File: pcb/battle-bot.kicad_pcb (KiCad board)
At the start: 4 copper layers, 99.2 x 51.2 mm, 219 parts, among them J1 Conn_01x02_Pin, J2 Conn_01x04_MountingPin, Q1 AON7544, Q2 AO3401A, Q21 GANE3R9, Q22 GANE3R9, Q23 GANE3R9, Q24 GANE3R9, Q25 GANE3R9, Q26 GANE3R9, Q27 AON7544, Q28 AON7544, Q29 AON7544, Q30 AON7544, Q31 AON7544, Q32 AON7544, Q33 AON7544, Q34 AON7544, Q35 AON7544, Q36 AON7544, Q37 AON7544, Q38 AON7544, Q39 AON7544, Q40 AON7544, Q41 AON7544, Q42 AON7544, Q43 AON7544, U1 TPS53319, U10 LMG1205, U11 LMG1205, U12 LMG1205, U13 ACS780xLRTR-100B, U15 LP38690SD, U2 nRF24L01P, U3 AT2401C, U4 ICM-42688-P, U5 LFL152G45TC1A219, U6 STM32G431RBTx, U7 DRV8323H, U8 DRV8323H, U9 DRV8323H, Y1 16MHz

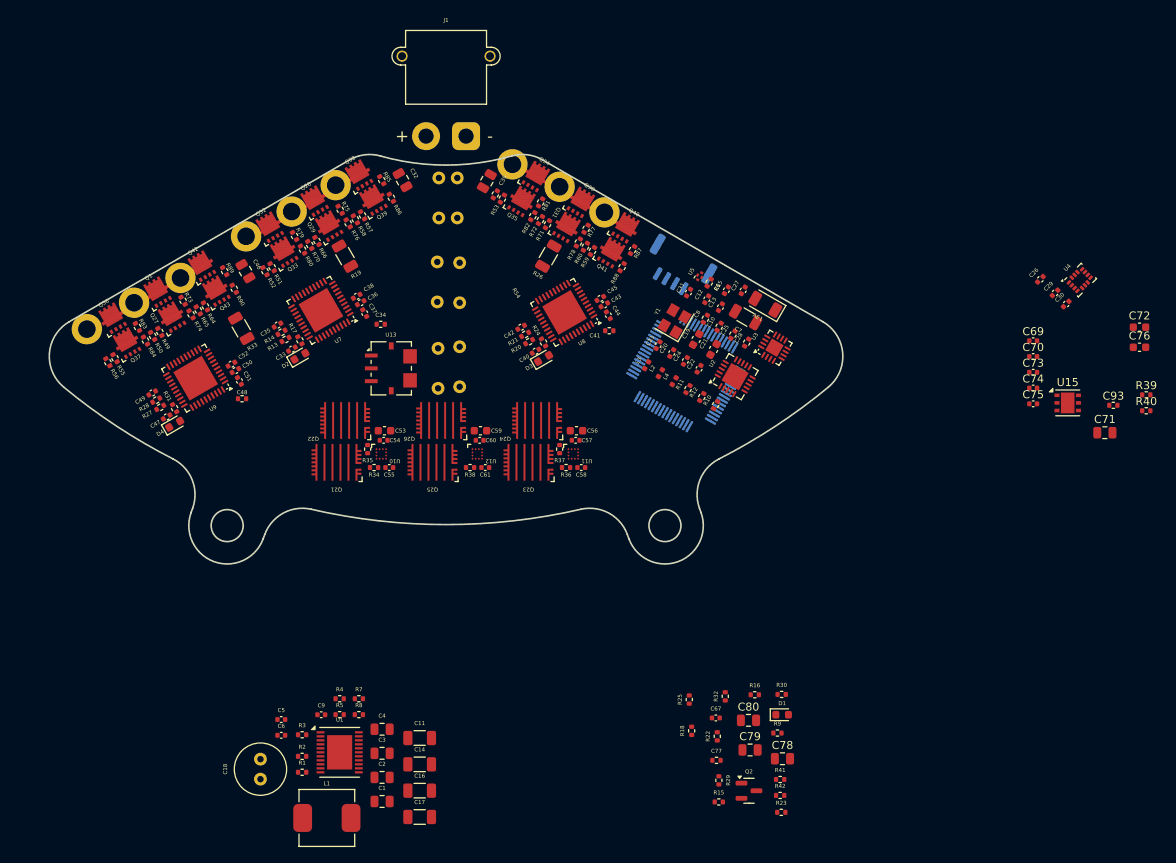
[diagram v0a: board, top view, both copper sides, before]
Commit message: Save layout
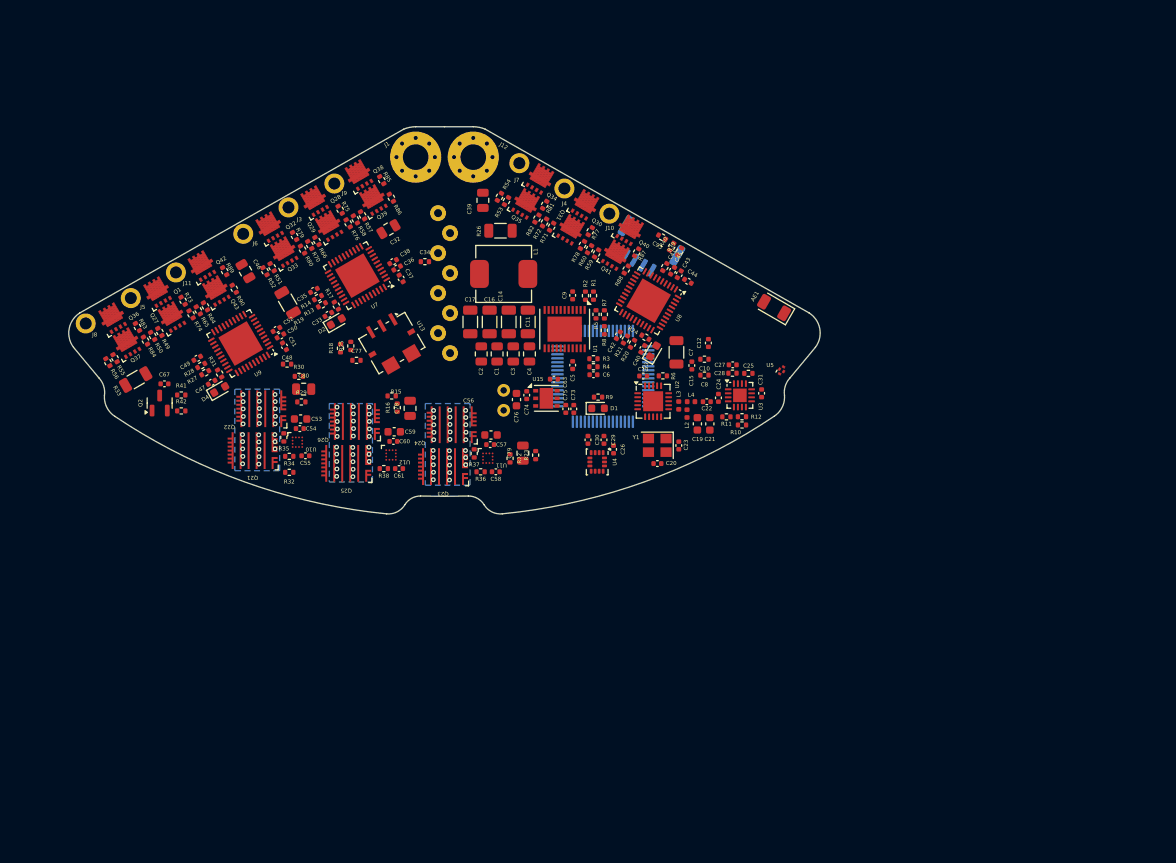
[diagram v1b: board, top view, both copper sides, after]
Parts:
- removed ? (x3): , 
- removed the C68 at (99.2, 54.9)
- removed the C68 at (99.1, 44.1)
- removed the C68 at (101.9, 49.2)
- removed the C68 at (101.9, 59.7)
- removed the C68 at (99.3, 33.6)
- removed C69, C70: 100n, Capacitor_SMD:C_0402_1005Metric
- removed C71: 22u, Capacitor_SMD:C_0805_2012Metric
- removed C72: 22u, Capacitor_SMD:C_0603_1608Metric
- removed REF** (x6): MountingHole_2.2mm_M2_DIN965_Pad, MountingHole:MountingHole_2.2mm_M2_DIN965_Pad
- added C62: 2m2, User_Footprints:C_D10xL16_Horizontal, B.Cu at (100.7, 40.5)
- added C63: 100n, Capacitor_SMD:C_0402_1005Metric, F.Cu at (113.7, 58.8)
- added C65: 2m2, User_Footprints:C_D10xL16_Horizontal, B.Cu at (99.2, 53.0)
- added C66: 2m2, User_Footprints:C_D10xL16_Horizontal, B.Cu at (100.7, 50.5)
- added J10: Conn_01x01_Pin, User_Footprints:Pad-P1.5, F.Cu at (120.6, 38.1)
- added J11: Conn_01x01_Pin, User_Footprints:Pad-P1.5, F.Cu at (66.4, 45.4)
- added J12: Conn_01x01_Pin, MountingHole:MountingHole_3.2mm_M3_Pad_Via, F.Cu at (103.6, 31.0)
- added J3: Conn_01x01_Pin, User_Footprints:Pad-P1.5, F.Cu at (80.5, 37.3)
- added J4: Conn_01x01_Pin, User_Footprints:Pad-P1.5, F.Cu at (115.0, 34.9)
- added J5: Conn_01x01_Pin, User_Footprints:Pad-P1.5, F.Cu at (60.8, 48.6)
- added J6: Conn_01x01_Pin, User_Footprints:Pad-P1.5, F.Cu at (74.8, 40.6)
- added J7: Conn_01x01_Pin, User_Footprints:Pad-P1.5, F.Cu at (109.4, 31.8)
- added J8: Conn_01x01_Pin, User_Footprints:Pad-P1.5, F.Cu at (55.2, 51.8)
- added J9: Conn_01x01_Pin, User_Footprints:Pad-P1.5, F.Cu at (86.2, 34.3)
- AE1: value Antenna -> Antenna_Chip
- C18: moved to B.Cu
- C68: footprint Capacitor_THT:C_Radial_D10.0mm_H16.0mm_P5.00mm -> User_Footprints:C_D10xL16_Horizontal
- J1: value Conn_01x02_Pin -> Conn_01x01_Pin; footprint Connector_AMASS:AMASS_XT30PW-M_1x02_P2.50mm_Horizontal -> MountingHole:MountingHole_3.2mm_M3_Pad_Via
- moved R41 89.0 mm to (67.1, 60.7)
- moved R42 89.0 mm to (67.1, 62.7)
- moved Q2 88.2 mm to (64.4, 61.7), turned to 90 degrees
- moved C67 80.6 mm to (65.0, 59.3)
- moved C76 78.2 mm to (109.0, 61.3), turned to -90 degrees
- moved R30 72.3 mm to (81.8, 58.4)
- moved L1 71.5 mm to (107.4, 45.6), turned to 180 degrees
- moved R29 70.4 mm to (82.1, 61.6), turned to 0 degrees
- moved R1 69.8 mm to (118.6, 48.3), turned to 90 degrees
- moved C80 69.3 mm to (82.4, 60.0)
- moved R2 67.6 mm to (117.6, 48.3), turned to -90 degrees
- moved C77 67.3 mm to (89.0, 56.4)
- moved R15 65.2 mm to (93.4, 60.9), turned to 180 degrees
- moved U15 65.2 mm to (112.7, 61.1)
- moved R18 64.9 mm to (87.0, 54.9)
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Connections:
- AE1 pad 2: (no net) -> unconnected-(AE1-PCB_Trace-Pad2)
- C68 pad 1: VDD -> GND
- C68 pad 2: GND -> VDD
- J1 pad 1: VDD -> GND
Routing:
- net /LargeMotor/OUTC: vias 0 -> 28
- net /LargeMotor/OUTB: vias 0 -> 28
- net /LargeMotor/OUTA: vias 0 -> 28
- added copper zone on B.Cu, net /LargeMotor/OUTA
- added copper zone on B.Cu, net /LargeMotor/OUTB
- added copper zone on B.Cu, net /LargeMotor/OUTC
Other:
- board size 99.2 x 51.2 mm -> 93.9 x 48.4 mm
- board text added: "Please Don't Explode 9000"

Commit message: Save old buck regulator
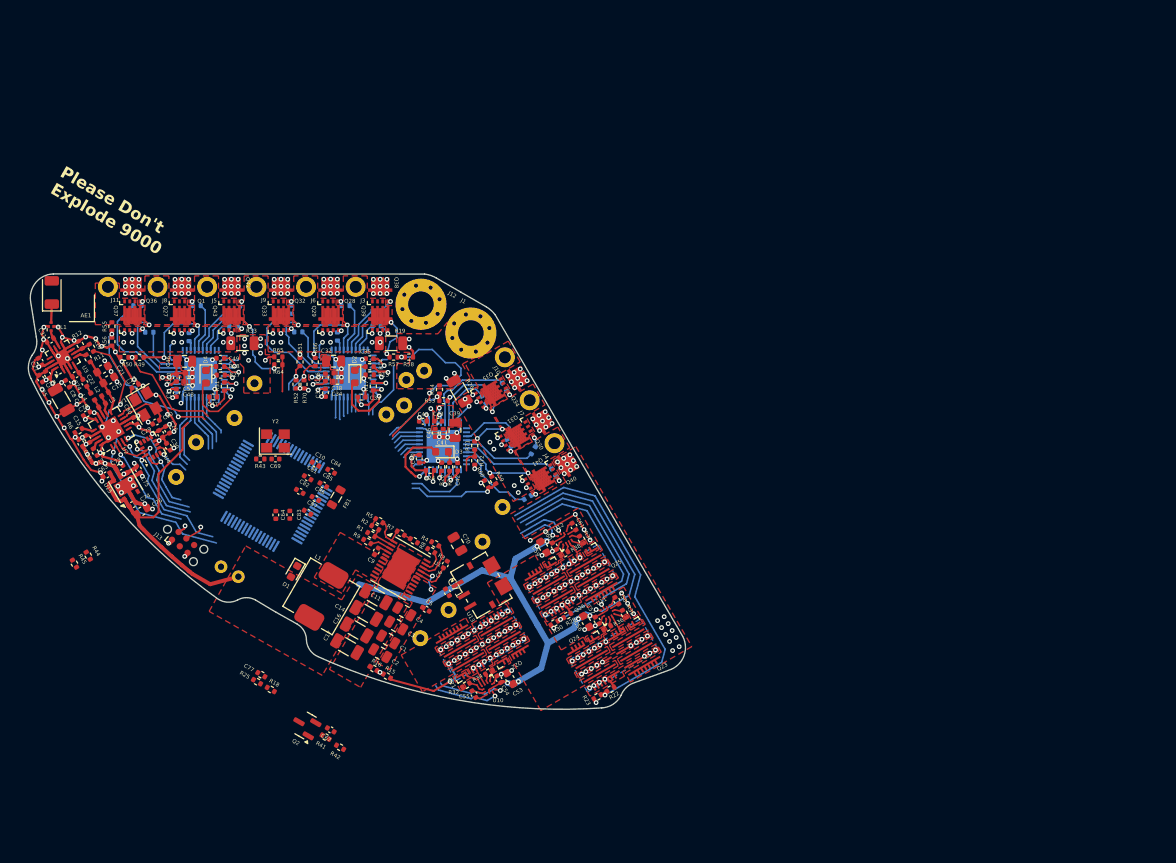
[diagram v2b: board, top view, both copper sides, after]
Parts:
- removed C93: 10u, Resistor_SMD:R_0402_1005Metric
- removed J2: Conn_01x04_MountingPin, Connector_JST:JST_GH_SM04B-GHS-TB_1x04-1MP_P1.25mm_Horizontal
- removed R39, R40: 2k2, Resistor_SMD:R_0402_1005Metric
- added C64: 12p, Capacitor_SMD:C_0402_1005Metric, F.Cu at (78.9, 75.7)
- added C69: 12p, Capacitor_SMD:C_0402_1005Metric, F.Cu at (78.9, 68.7)
- added C70: 22u, Capacitor_SMD:C_0805_2012Metric, F.Cu at (101.6, 79.3)
- added C71: 100n, Capacitor_SMD:C_0402_1005Metric, F.Cu at (100.4, 85.4)
- added C72: 2m2, User_Footprints:C_D10xL16_Horizontal, B.Cu at (104.7, 79.1)
- added C81: 100n, Capacitor_SMD:C_0402_1005Metric, F.Cu at (82.9, 71.1)
- added C82: 100n, Capacitor_SMD:C_0402_1005Metric, F.Cu at (81.9, 72.8)
- added C83: 100n, Capacitor_SMD:C_0402_1005Metric, F.Cu at (80.7, 75.7)
- added C84: 100n, Capacitor_SMD:C_0402_1005Metric, F.Cu at (85.8, 70.3)
- added C85: 1u, Capacitor_SMD:C_0402_1005Metric, F.Cu at (84.8, 72.0)
- added C86: 1u, Capacitor_SMD:C_0402_1005Metric, F.Cu at (83.9, 73.7)
- added C87: 100n, Capacitor_SMD:C_0402_1005Metric, F.Cu at (82.9, 75.4)
- added FB1: FerriteBead, Inductor_SMD:L_0805_2012Metric, F.Cu at (86.5, 73.5)
- added J13: Conn_ARM_SWD_TagConnect_TC2030-NL, Connector:Tag-Connect_TC2030-IDC-NL_2x03_P1.27mm_Vertical, F.Cu at (67.3, 79.2)
- added R43: 1k, Resistor_SMD:R_0402_1005Metric, F.Cu at (77.0, 68.7)
- added R44: 15k, Resistor_SMD:R_0402_1005Metric, F.Cu at (55.5, 80.8)
- added R45: 2k2, Resistor_SMD:R_0402_1005Metric, F.Cu at (53.7, 81.8)
- added Y2: 16MHz, Crystal:Crystal_SMD_3225-4Pin_3.2x2.5mm, F.Cu at (78.9, 66.5)
- C10: value 100n -> 10u; footprint Resistor_SMD:R_0402_1005Metric -> Capacitor_SMD:C_0402_1005Metric
- C25, C28: footprint Resistor_SMD:R_0402_1005Metric -> Capacitor_SMD:C_0402_1005Metric
- C67: value C -> 4u7
- C7: footprint Resistor_SMD:R_1206_3216Metric -> Capacitor_SMD:C_1206_3216Metric
- C78: value 22u -> 2m2; footprint Capacitor_SMD:C_0805_2012Metric -> User_Footprints:C_D10xL16_Horizontal; moved to B.Cu
- C79, C80: value 22u -> 10n; footprint Capacitor_SMD:C_0805_2012Metric -> Capacitor_SMD:C_0402_1005Metric
- C8: value 10u -> 1u; footprint Resistor_SMD:R_0402_1005Metric -> Capacitor_SMD:C_0402_1005Metric
- R1: value 22k -> 47k
- R15, R22, R29: value 4k7 -> 10k
- R16, R23, R30: value 1k -> 1k5
- R2: value 10k -> 4k7
- R42: value R -> 100k
- R73, R74, R75, R76, R77, R78, R79, R80, R81, R82, R83, R84, R85, R86, R87, R88, R89, R90, U7, U8, U9: moved to B.Cu
- moved FL1 91.5 mm to (50.8, 52.2), turned to 90 degrees
- moved AE1 90.3 mm to (50.9, 47.9), turned to 90 degrees
- moved C31 89.2 mm to (50.7, 53.9), turned to -150 degrees
- moved C25 88.5 mm to (49.5, 58.7), turned to 120 degrees
- moved C27 86.6 mm to (49.5, 56.6), turned to 120 degrees
- moved C28 85.6 mm to (50.4, 58.2), turned to 120 degrees
- moved U3 84.8 mm to (52.3, 56.0), turned to 120 degrees
- moved R12 83.2 mm to (54.5, 54.5), turned to 120 degrees
- moved R10 81.9 mm to (55.9, 54.8), turned to -60 degrees
- moved C24 80.4 mm to (53.9, 58.2), turned to -150 degrees
- moved R11 80.1 mm to (55.5, 56.1), turned to 120 degrees
- moved C8 79.6 mm to (52.9, 59.3), turned to -60 degrees
- moved C12 79.4 mm to (54.5, 66.7), turned to 120 degrees
- moved C22 77.8 mm to (55.0, 59.2), turned to 120 degrees
- moved C7 77.1 mm to (52.1, 61.4), turned to -60 degrees
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- renumbered U5 to FL1
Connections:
- C35 pad 1: Net-(U7-VREF) -> +3V3
- C42 pad 1: Net-(U8-VREF) -> +3V3
- C49 pad 1: Net-(U9-VREF) -> +3V3
- C73 pad 1: VDDRF -> +3V3
- C75 pad 1: VDDRF -> +3V3
- C79 pad 1: VDD -> +3V3
- C80 pad 1: VDD -> +3V3
- Q1 pad 1: /SmallMotor3/OUTA -> /SmallMotor3/OUTB
- Q1 pad 2: /SmallMotor3/OUTA -> /SmallMotor3/OUTB
- Q1 pad 3: /SmallMotor3/OUTA -> /SmallMotor3/OUTB
- Q27 pad 5: /SmallMotor3/OUTA -> /SmallMotor3/OUTB
- Q27 pad 6: /SmallMotor3/OUTA -> /SmallMotor3/OUTB
- Q27 pad 7: /SmallMotor3/OUTA -> /SmallMotor3/OUTB
- Q27 pad 8: /SmallMotor3/OUTA -> /SmallMotor3/OUTB
- Q28 pad 1: /SmallMotor1/OUTA -> /SmallMotor1/OUTB
- Q28 pad 2: /SmallMotor1/OUTA -> /SmallMotor1/OUTB
- Q28 pad 3: /SmallMotor1/OUTA -> /SmallMotor1/OUTB
- Q29 pad 5: /SmallMotor1/OUTA -> /SmallMotor1/OUTB
- Q29 pad 6: /SmallMotor1/OUTA -> /SmallMotor1/OUTB
- Q29 pad 7: /SmallMotor1/OUTA -> /SmallMotor1/OUTB
- Q29 pad 8: /SmallMotor1/OUTA -> /SmallMotor1/OUTB
- Q30 pad 1: /SmallMotor2/OUTA -> /SmallMotor2/OUTB
- Q30 pad 2: /SmallMotor2/OUTA -> /SmallMotor2/OUTB
- Q30 pad 3: /SmallMotor2/OUTA -> /SmallMotor2/OUTB
- Q31 pad 5: /SmallMotor2/OUTA -> /SmallMotor2/OUTB
- Q31 pad 6: /SmallMotor2/OUTA -> /SmallMotor2/OUTB
- Q31 pad 7: /SmallMotor2/OUTA -> /SmallMotor2/OUTB
- Q31 pad 8: /SmallMotor2/OUTA -> /SmallMotor2/OUTB
- Q32 pad 1: /SmallMotor1/OUTB -> /SmallMotor1/OUTC
- Q32 pad 2: /SmallMotor1/OUTB -> /SmallMotor1/OUTC
- Q32 pad 3: /SmallMotor1/OUTB -> /SmallMotor1/OUTC
- Q33 pad 5: /SmallMotor1/OUTB -> /SmallMotor1/OUTC
- Q33 pad 6: /SmallMotor1/OUTB -> /SmallMotor1/OUTC
- Q33 pad 7: /SmallMotor1/OUTB -> /SmallMotor1/OUTC
- Q33 pad 8: /SmallMotor1/OUTB -> /SmallMotor1/OUTC
- Q34 pad 1: /SmallMotor2/OUTB -> /SmallMotor2/OUTC
- Q34 pad 2: /SmallMotor2/OUTB -> /SmallMotor2/OUTC
- Q34 pad 3: /SmallMotor2/OUTB -> /SmallMotor2/OUTC
- Q35 pad 5: /SmallMotor2/OUTB -> /SmallMotor2/OUTC
- Q35 pad 6: /SmallMotor2/OUTB -> /SmallMotor2/OUTC
- Q35 pad 7: /SmallMotor2/OUTB -> /SmallMotor2/OUTC
- Q35 pad 8: /SmallMotor2/OUTB -> /SmallMotor2/OUTC
- Q36 pad 1: /SmallMotor3/OUTB -> /SmallMotor3/OUTC
- Q36 pad 2: /SmallMotor3/OUTB -> /SmallMotor3/OUTC
- Q36 pad 3: /SmallMotor3/OUTB -> /SmallMotor3/OUTC
- Q37 pad 5: /SmallMotor3/OUTB -> /SmallMotor3/OUTC
- Q37 pad 6: /SmallMotor3/OUTB -> /SmallMotor3/OUTC
- Q37 pad 7: /SmallMotor3/OUTB -> /SmallMotor3/OUTC
- Q37 pad 8: /SmallMotor3/OUTB -> /SmallMotor3/OUTC
- Q38 pad 1: /SmallMotor1/OUTC -> /SmallMotor1/OUTA
- Q38 pad 2: /SmallMotor1/OUTC -> /SmallMotor1/OUTA
- Q38 pad 3: /SmallMotor1/OUTC -> /SmallMotor1/OUTA
- Q39 pad 5: /SmallMotor1/OUTC -> /SmallMotor1/OUTA
- Q39 pad 6: /SmallMotor1/OUTC -> /SmallMotor1/OUTA
- Q39 pad 7: /SmallMotor1/OUTC -> /SmallMotor1/OUTA
- Q39 pad 8: /SmallMotor1/OUTC -> /SmallMotor1/OUTA
- Q40 pad 1: /SmallMotor2/OUTC -> /SmallMotor2/OUTA
- Q40 pad 2: /SmallMotor2/OUTC -> /SmallMotor2/OUTA
- Q40 pad 3: /SmallMotor2/OUTC -> /SmallMotor2/OUTA
- Q41 pad 5: /SmallMotor2/OUTC -> /SmallMotor2/OUTA
- Q41 pad 6: /SmallMotor2/OUTC -> /SmallMotor2/OUTA
- Q41 pad 7: /SmallMotor2/OUTC -> /SmallMotor2/OUTA
- Q41 pad 8: /SmallMotor2/OUTC -> /SmallMotor2/OUTA
- Q42 pad 1: /SmallMotor3/OUTC -> /SmallMotor3/OUTA
- Q42 pad 2: /SmallMotor3/OUTC -> /SmallMotor3/OUTA
- Q42 pad 3: /SmallMotor3/OUTC -> /SmallMotor3/OUTA
- Q43 pad 5: /SmallMotor3/OUTC -> /SmallMotor3/OUTA
- Q43 pad 6: /SmallMotor3/OUTC -> /SmallMotor3/OUTA
- Q43 pad 7: /SmallMotor3/OUTC -> /SmallMotor3/OUTA
- Q43 pad 8: /SmallMotor3/OUTC -> /SmallMotor3/OUTA
- R10 pad 2: /CE -> /RCE
- R15 pad 1: /LargeMotor/OUTA -> /WCPA
- R15 pad 2: /WCPB -> /LargeMotor/OUTA
- R16 pad 1: /WCPB -> /WCPA
- R22 pad 1: /LargeMotor/OUTB -> /WCPB
- R22 pad 2: /WCPB -> /LargeMotor/OUTB
- R29 pad 1: /LargeMotor/OUTC -> /WCPC
- R29 pad 2: /WCPC -> /LargeMotor/OUTC
- R49 pad 1: /SmallMotor3/OUTA -> /SmallMotor3/OUTB
- R49 pad 2: /CPA3 -> /CPB3
- R50 pad 1: /CPA3 -> /CPB3
- R51 pad 1: /SmallMotor1/OUTB -> /SmallMotor1/OUTC
- R51 pad 2: /CPB1 -> /CPC1
- R52 pad 1: /CPB1 -> /CPC1
- R53 pad 1: /SmallMotor2/OUTB -> /SmallMotor2/OUTC
- R53 pad 2: /CPB2 -> /CPC2
- R54 pad 1: /CPB2 -> /CPC2
- R55 pad 1: /SmallMotor3/OUTB -> /SmallMotor3/OUTC
- R55 pad 2: /CPB3 -> /CPC3
- R56 pad 1: /CPB3 -> /CPC3
- R57 pad 1: /SmallMotor1/OUTC -> /SmallMotor1/OUTA
- R57 pad 2: /CPC1 -> /CPA1
- R58 pad 1: /CPC1 -> /CPA1
- R59 pad 1: /SmallMotor2/OUTC -> /SmallMotor2/OUTA
- R59 pad 2: /CPC2 -> /CPA2
- R60 pad 1: /CPC2 -> /CPA2
- R64 pad 1: /SmallMotor3/OUTC -> /SmallMotor3/OUTA
- R64 pad 2: /CPC3 -> /CPA3
- R65 pad 1: /CPC3 -> /CPA3
- R66 pad 1: /SmallMotor1/OUTA -> /SmallMotor1/OUTB
- R66 pad 2: /CPA1 -> /CPB1
- R70 pad 1: /CPA1 -> /CPB1
- R71 pad 1: /SmallMotor2/OUTA -> /SmallMotor2/OUTB
- R71 pad 2: /CPA2 -> /CPB2
- R72 pad 1: /CPA2 -> /CPB2
- R73 pad 1: /SmallMotor3/GHA -> /SmallMotor3/GHB
- R74 pad 1: /SmallMotor3/GLA -> /SmallMotor3/GLB
- R75 pad 1: /SmallMotor1/GHA -> /SmallMotor1/GHB
- R76 pad 1: /SmallMotor1/GLA -> /SmallMotor1/GLB
- R77 pad 1: /SmallMotor2/GHA -> /SmallMotor2/GHB
- R78 pad 1: /SmallMotor2/GLA -> /SmallMotor2/GLB
- R79 pad 1: /SmallMotor1/GHB -> /SmallMotor1/GHC
- R80 pad 1: /SmallMotor1/GLB -> /SmallMotor1/GLC
- R81 pad 1: /SmallMotor2/GHB -> /SmallMotor2/GHC
- R82 pad 1: /SmallMotor2/GLB -> /SmallMotor2/GLC
- R83 pad 1: /SmallMotor3/GHB -> /SmallMotor3/GHC
- R84 pad 1: /SmallMotor3/GLB -> /SmallMotor3/GLC
- R85 pad 1: /SmallMotor1/GHC -> /SmallMotor1/GHA
- R86 pad 1: /SmallMotor1/GLC -> /SmallMotor1/GLA
- R87 pad 1: /SmallMotor2/GHC -> /SmallMotor2/GHA
- R88 pad 1: /SmallMotor2/GLC -> /SmallMotor2/GLA
- R89 pad 1: /SmallMotor3/GHC -> /SmallMotor3/GHA
- R90 pad 1: /SmallMotor3/GLC -> /SmallMotor3/GLA
- U15 pad 4: VDDRF -> +3V3
- U15 pad 5: VDDRF -> +3V3
- U6 pad 1: unconnected-(U6-VBAT-Pad1) -> /VBAT
- U6 pad 10: unconnected-(U6-PC2-Pad10) -> /WHC
- U6 pad 11: unconnected-(U6-PC3-Pad11) -> /CPB3
- U6 pad 12: unconnected-(U6-PA0-Pad12) -> /SO1
- U6 pad 13: unconnected-(U6-PA1-Pad13) -> /SO2
- U6 pad 14: unconnected-(U6-PA2-Pad14) -> /SO3
- U6 pad 16: unconnected-(U6-VDD-Pad16) -> +3V3
- U6 pad 17: unconnected-(U6-PA3-Pad17) -> /WSO
- U6 pad 18: unconnected-(U6-PA4-Pad18) -> /WCPA
- U6 pad 19: unconnected-(U6-PA5-Pad19) -> /WCPB
- U6 pad 2: unconnected-(U6-PC13-Pad2) -> /WLA
- U6 pad 20: unconnected-(U6-PA6-Pad20) -> /WCPC
- U6 pad 21: unconnected-(U6-PA7-Pad21) -> /CPA2
- U6 pad 22: unconnected-(U6-PC4-Pad22) -> /CPB2
- U6 pad 23: unconnected-(U6-PC5-Pad23) -> /CPC2
- U6 pad 24: unconnected-(U6-PB0-Pad24) -> /WLB
- U6 pad 25: unconnected-(U6-PB1-Pad25) -> /WLC
- U6 pad 26: unconnected-(U6-PB2-Pad26) -> /CPA3
- U6 pad 28: unconnected-(U6-VREF+-Pad28) -> +3V3A
- U6 pad 29: unconnected-(U6-VDDA-Pad29) -> +3V3A
- U6 pad 3: unconnected-(U6-PC14-Pad3) -> /GINT
- U6 pad 30: unconnected-(U6-PB10-Pad30) -> /INHC1
- U6 pad 32: unconnected-(U6-VDD-Pad32) -> +3V3
- U6 pad 33: unconnected-(U6-PB11-Pad33) -> /CPC3
- U6 pad 34: unconnected-(U6-PB12-Pad34) -> /CPA1
- U6 pad 35: unconnected-(U6-PB13-Pad35) -> /CLK
- U6 pad 36: unconnected-(U6-PB14-Pad36) -> /CPB1
- U6 pad 37: unconnected-(U6-PB15-Pad37) -> /CPC1
- U6 pad 38: unconnected-(U6-PC6-Pad38) -> /INHA2
- U6 pad 39: unconnected-(U6-PC7-Pad39) -> /INHB2
- U6 pad 4: unconnected-(U6-PC15-Pad4) -> /INLB3
- U6 pad 40: unconnected-(U6-PC8-Pad40) -> /INHC2
- U6 pad 41: unconnected-(U6-PC9-Pad41) -> /INLA1
- U6 pad 42: unconnected-(U6-PA8-Pad42) -> /RCS
- U6 pad 43: unconnected-(U6-PA9-Pad43) -> /GCS
- U6 pad 44: unconnected-(U6-PA10-Pad44) -> /MISO
- U6 pad 45: unconnected-(U6-PA11-Pad45) -> /MOSI
- U6 pad 46: unconnected-(U6-PA12-Pad46) -> /RCE
- U6 pad 48: unconnected-(U6-VDD-Pad48) -> +3V3
- U6 pad 49: unconnected-(U6-PA13-Pad49) -> /SWDIO
- U6 pad 5: unconnected-(U6-PF0-Pad5) -> /XTO
- U6 pad 50: unconnected-(U6-PA14-Pad50) -> /SWCLK
- U6 pad 51: unconnected-(U6-PA15-Pad51) -> /INLC3
- U6 pad 52: unconnected-(U6-PC10-Pad52) -> /INLB2
- U6 pad 53: unconnected-(U6-PC11-Pad53) -> /INLC1
- U6 pad 54: unconnected-(U6-PC12-Pad54) -> /INLC2
- U6 pad 55: unconnected-(U6-PD2-Pad55) -> /INLA3
- U6 pad 56: unconnected-(U6-PB3-Pad56) -> /INHB1
- U6 pad 57: unconnected-(U6-PB4-Pad57) -> /INLA2
- U6 pad 58: unconnected-(U6-PB5-Pad58) -> /INHA1
- U6 pad 59: unconnected-(U6-PB6-Pad59) -> /INHA3
- U6 pad 6: unconnected-(U6-PF1-Pad6) -> /XTI
- U6 pad 60: unconnected-(U6-PB7-Pad60) -> /INHB3
- U6 pad 61: unconnected-(U6-PB8-Pad61) -> /INHC3
- U6 pad 62: unconnected-(U6-PB9-Pad62) -> /INLB1
- U6 pad 64: unconnected-(U6-VDD-Pad64) -> +3V3
- U6 pad 7: unconnected-(U6-PG10-Pad7) -> /RIRQ
- U6 pad 8: unconnected-(U6-PC0-Pad8) -> /WHA
- U6 pad 9: unconnected-(U6-PC1-Pad9) -> /WHB
- U7 pad 16: /SmallMotor1/GHC -> /SmallMotor1/GHA
- U7 pad 17: /SmallMotor1/OUTC -> /SmallMotor1/OUTA
- U7 pad 18: /SmallMotor1/GLC -> /SmallMotor1/GLA
- U7 pad 24: Net-(U7-VREF) -> +3V3
- U7 pad 6: /SmallMotor1/GHA -> /SmallMotor1/GHC
- U7 pad 7: /SmallMotor1/OUTA -> /SmallMotor1/OUTC
- U7 pad 8: /SmallMotor1/GLA -> /SmallMotor1/GLC
- U8 pad 16: /SmallMotor2/GHC -> /SmallMotor2/GHA
- U8 pad 17: /SmallMotor2/OUTC -> /SmallMotor2/OUTA
- U8 pad 18: /SmallMotor2/GLC -> /SmallMotor2/GLA
- U8 pad 24: Net-(U8-VREF) -> +3V3
- U8 pad 6: /SmallMotor2/GHA -> /SmallMotor2/GHC
- U8 pad 7: /SmallMotor2/OUTA -> /SmallMotor2/OUTC
- U8 pad 8: /SmallMotor2/GLA -> /SmallMotor2/GLC
- U9 pad 16: /SmallMotor3/GHC -> /SmallMotor3/GHA
- U9 pad 17: /SmallMotor3/OUTC -> /SmallMotor3/OUTA
- U9 pad 18: /SmallMotor3/GLC -> /SmallMotor3/GLA
- U9 pad 24: Net-(U9-VREF) -> +3V3
- U9 pad 6: /SmallMotor3/GHA -> /SmallMotor3/GHC
- U9 pad 7: /SmallMotor3/OUTA -> /SmallMotor3/OUTC
- U9 pad 8: /SmallMotor3/GLA -> /SmallMotor3/GLC
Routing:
- net GND: track 0.00 -> 197.6 mm, vias 0 -> 104
- net +5V: track 0.00 -> 131.2 mm, vias 0 -> 9
- net +3V3: track 0.00 -> 89.0 mm, vias 0 -> 19
- net /WCPB: track 0.00 -> 44.0 mm, vias 0 -> 1
- net /RCE: track 0.00 -> 36.2 mm, vias 0 -> 2
- net /WLB: track 0.00 -> 29.1 mm, vias 0 -> 1
- net /WCPC: track 0.00 -> 28.5 mm, vias 0 -> 1
- net /WHB: track 0.00 -> 25.6 mm, vias 0 -> 1
- net /CPA1: track 0.00 -> 22.9 mm, vias 0 -> 2
- net /CPC3: track 0.00 -> 19.6 mm, vias 0 -> 2
- net /MOSI: track 0.00 -> 19.2 mm, vias 0 -> 2
- net /SmallMotor3/OUTA: track 0.00 -> 18.2 mm, vias 0 -> 2
- net /SmallMotor3/OUTB: track 0.00 -> 16.1 mm, vias 0 -> 2
- net VDD: track 0.00 -> 15.5 mm, vias 0 -> 99
- net /CLK: track 0.00 -> 15.0 mm, vias 0 -> 1
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- added copper zone on F.Cu, net +5V
- added copper zone on F.Cu, net /LargeMotor/LargeBridgeA/PL
- added copper zone on F.Cu, net /LargeMotor/OUTA
- added copper zone on F.Cu, net /LargeMotor/OUTB
- added copper zone on F.Cu, net /LargeMotor/OUTC
- added copper zone on F.Cu, net /SmallMotor1/OUTA
- added copper zone on F.Cu, net /SmallMotor1/OUTB
- added copper zone on F.Cu, net /SmallMotor1/OUTC
- added copper zone on F.Cu, net /SmallMotor1/SP
- added copper zone on In1.Cu, net /SmallMotor1/SP
- added copper zone on F.Cu, net /SmallMotor2/OUTA
- added copper zone on F.Cu, net /SmallMotor2/OUTB
- added copper zone on F.Cu, net /SmallMotor2/OUTC
- added copper zone on F.Cu, net /SmallMotor2/SP
- added copper zone on In1.Cu, net /SmallMotor2/SP
- added copper zone on F.Cu, net /SmallMotor3/OUTA
- added copper zone on F.Cu, net /SmallMotor3/OUTB
- added copper zone on F.Cu, net /SmallMotor3/OUTC
- added copper zone on F.Cu, net /SmallMotor3/SP
- added copper zone on In1.Cu, net /SmallMotor3/SP
- added copper zone on F.Cu, net GND
- added copper zone on F.Cu, net Net-(C9-Pad1)
- added copper zone on F.Cu, net Net-(U10-HOL)
- added copper zone on F.Cu, net Net-(U10-LOL)
- added copper zone on F.Cu, net Net-(U11-HOL)
- added copper zone on F.Cu, net Net-(U11-LOL)
- added copper zone on F.Cu, net Net-(U12-HOL)
- added copper zone on F.Cu, net Net-(U12-LOL)
- added copper zone on F.Cu, net VDD
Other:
- board size 93.9 x 48.4 mm -> 82.1 x 54.4 mm
